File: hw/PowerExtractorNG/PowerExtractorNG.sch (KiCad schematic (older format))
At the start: 11 parts, among them J1 INPUT RECTIFIED, J2 OUTPUT, Q1 IRFB4110

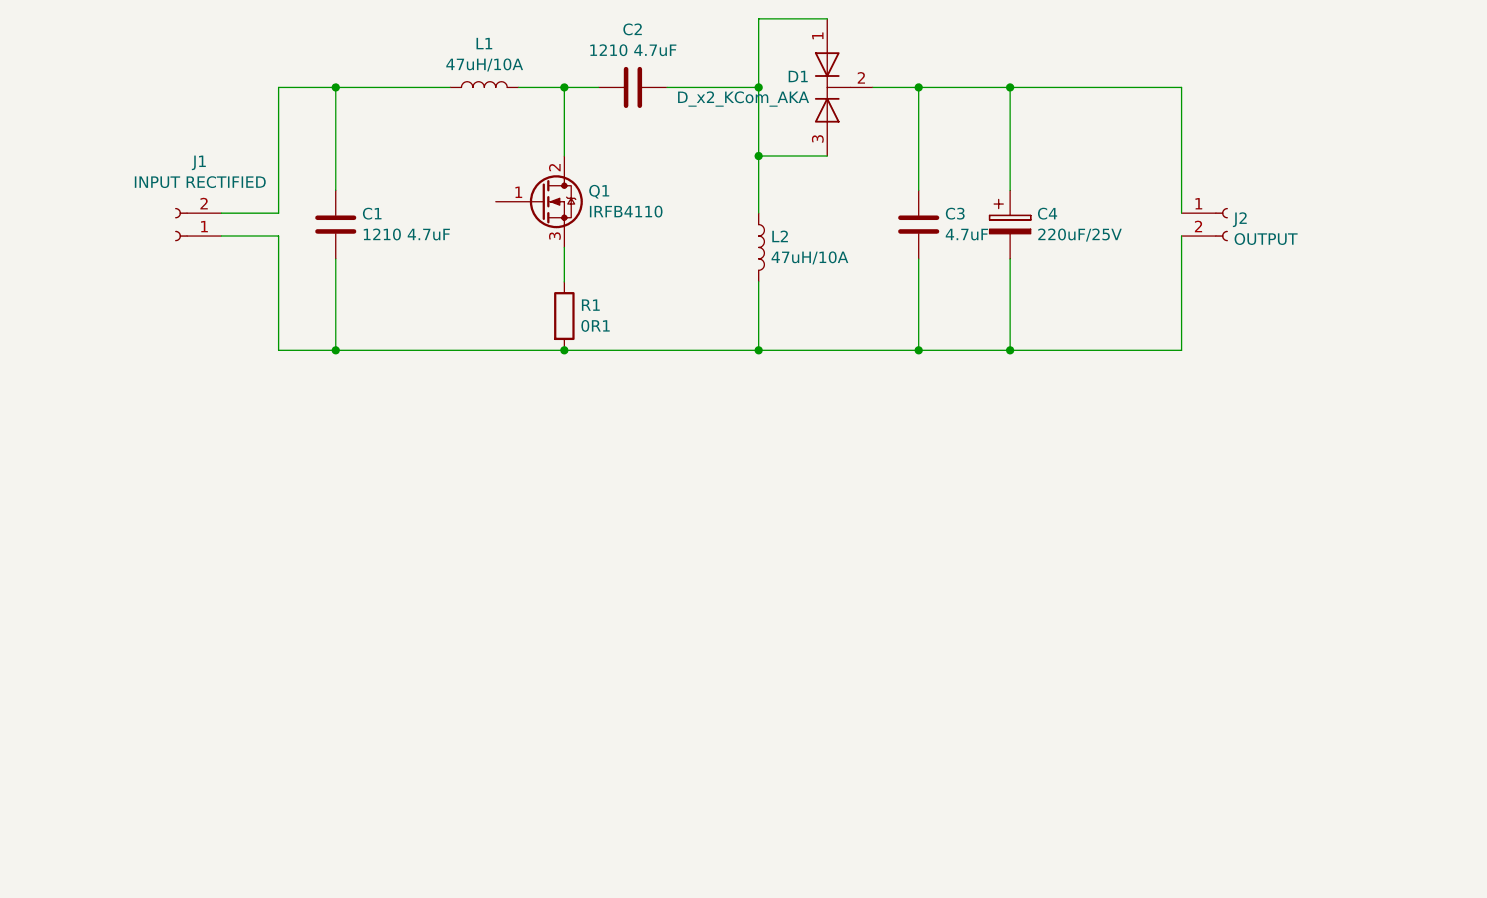
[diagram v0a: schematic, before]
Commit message: Done
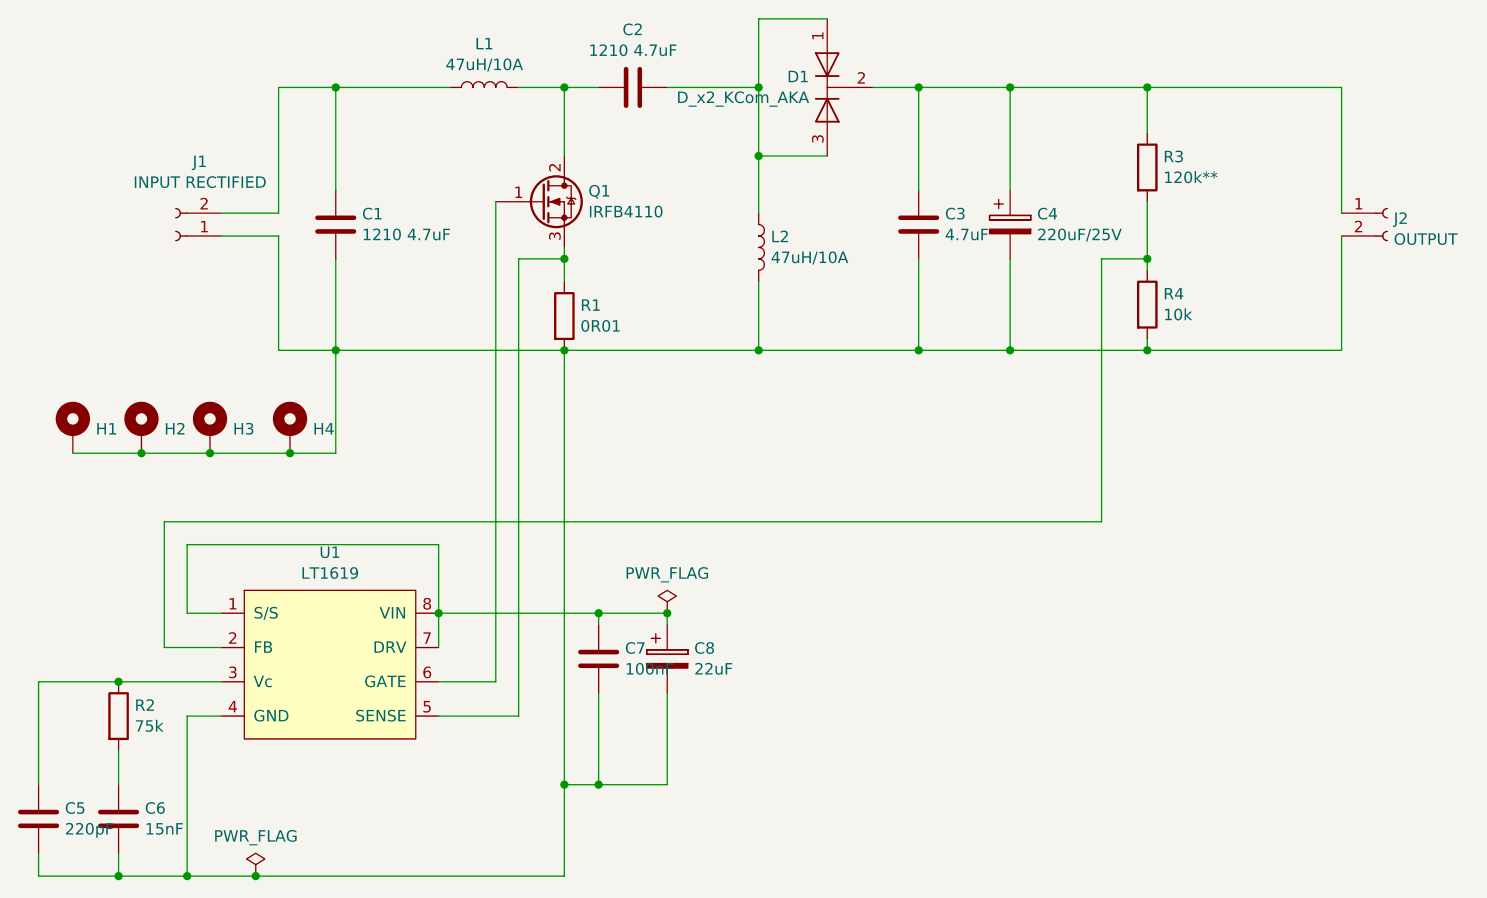
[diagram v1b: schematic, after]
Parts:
- added C5: 220pF, Capacitor_SMD:C_1206_3216Metric_Pad1.42x1.75mm_HandSolder, symbol Device:C
- added C6: 15nF, Capacitor_SMD:C_1206_3216Metric_Pad1.42x1.75mm_HandSolder, symbol Device:C
- added C7: 100nF, Capacitor_SMD:C_1206_3216Metric_Pad1.42x1.75mm_HandSolder, symbol Device:C
- added C8: 22uF, Capacitor_THT:CP_Radial_D7.5mm_P2.50mm, symbol Device:CP
- added H1, H2, H3, H4: MountingHole_Pad, MountingHole:MountingHole_3.2mm_M3_Pad, symbol Mechanical:MountingHole_Pad
- added R2: 75k, Resistor_SMD:R_1206_3216Metric_Pad1.42x1.75mm_HandSolder, symbol Device:R
- added R3: 120k**, Resistor_SMD:R_1206_3216Metric_Pad1.42x1.75mm_HandSolder, symbol Device:R
- added R4: 10k, Resistor_SMD:R_1206_3216Metric_Pad1.42x1.75mm_HandSolder, symbol Device:R
- added U1: LT1619, Package_SO:SO-8_5.3x6.2mm_P1.27mm, symbol triakcz_kicad:LT1619
- C4: footprint Capacitor_THT:C_Rect_L7.2mm_W5.5mm_P5.00mm_FKS2_FKP2_MKS2_MKP2 -> Capacitor_THT:CP_Radial_D10.0mm_P5.00mm
- R1: value 0R1 -> 0R01; footprint Resistor_SMD:R_1206_3216Metric_Pad1.42x1.75mm_HandSolder -> Resistor_SMD:R_2512_6332Metric_Pad1.52x3.35mm_HandSolder
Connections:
- net at C1.2, C3.2, C4.2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: now also C5.2, C6.2, C7.2, C8.2, H1.1, H2.1, H3.1, H4.1, R4.2, U1.4 (GND)
- net at C3.1, C4.1, D1.2 (K)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: now also R3.1
- net at Q1.1 (G): now also U1.6 (GATE)
- net at Q1.3 (S), R1.1: now also U1.5 (SENSE)
- new net: C7.1, C8.1, U1.1 (S/S), U1.7 (DRV), U1.8 (VIN)
- new net: R3.2, R4.1, U1.2 (FB)
- new net: C5.1, R2.1, U1.3 (Vc)
- new net: C6.1, R2.2
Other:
- moved on the sheet: J2

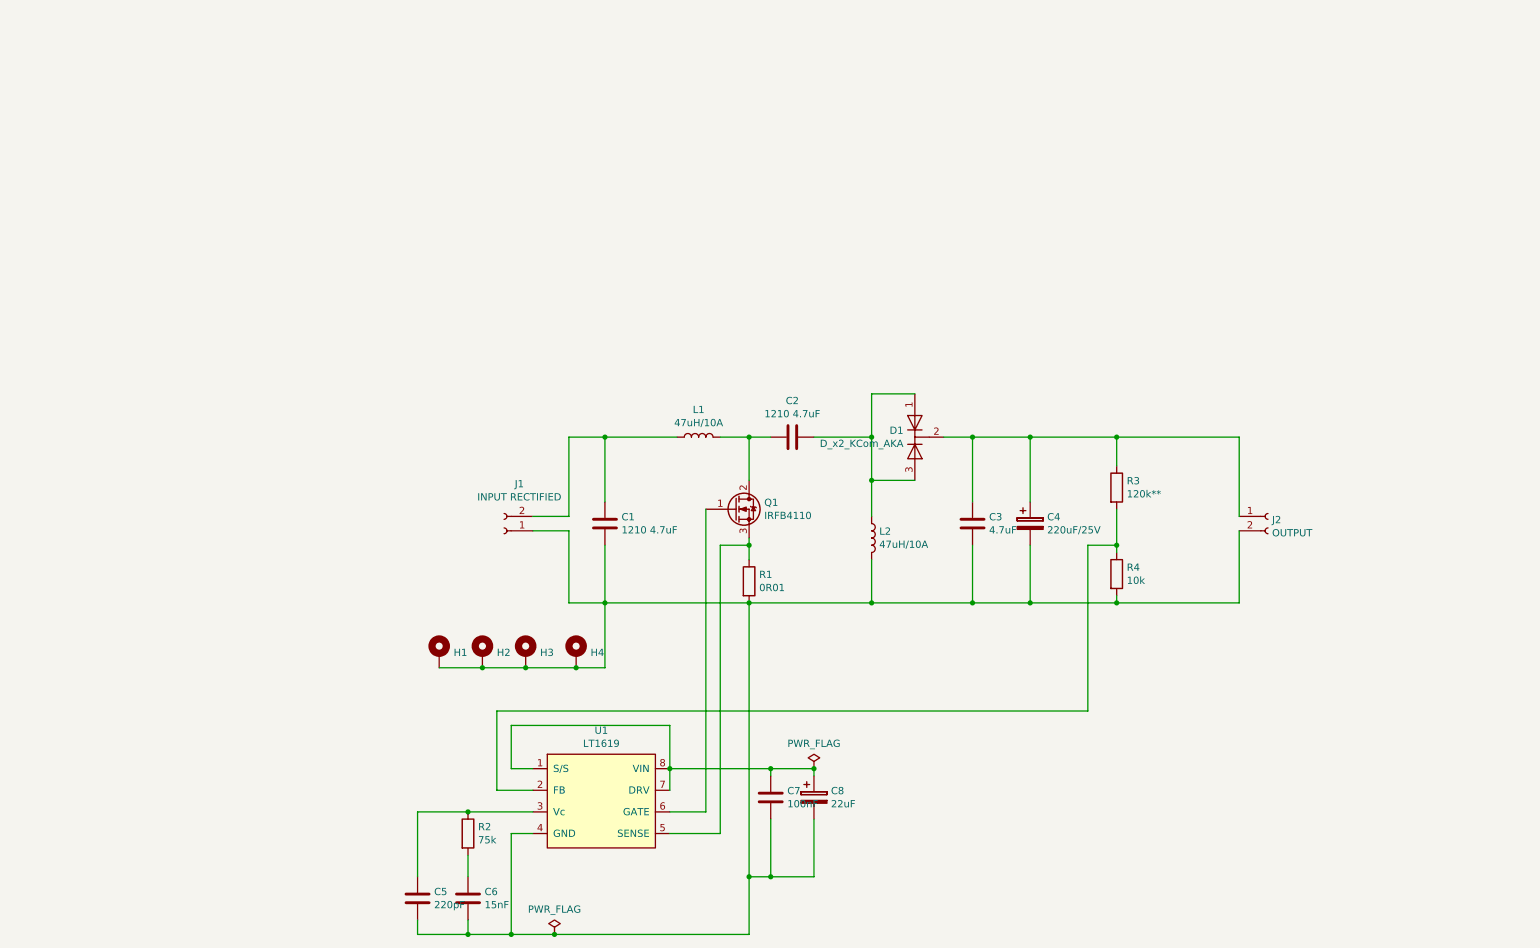
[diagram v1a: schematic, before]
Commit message: PE2020
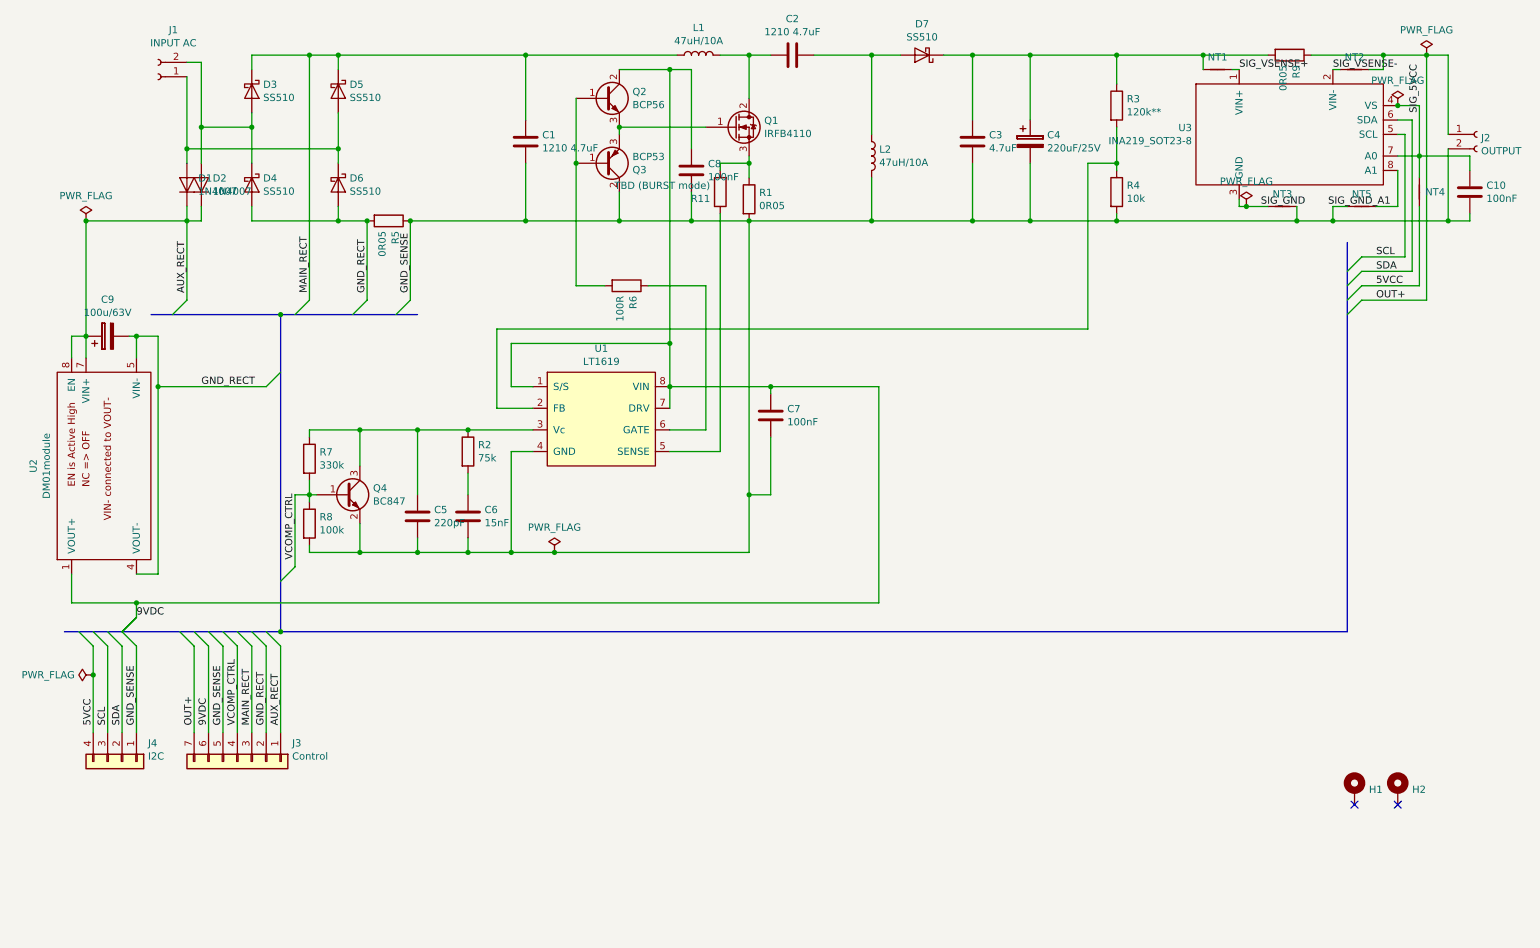
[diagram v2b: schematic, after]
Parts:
- removed C8: 22uF, Capacitor_THT:CP_Radial_D7.5mm_P2.50mm, symbol Device:CP
- removed D1: D_x2_KCom_AKA, Package_TO_SOT_THT:TO-220-3_Vertical, symbol Device:D_x2_KCom_AKA
- removed H3, H4: MountingHole_Pad, MountingHole:MountingHole_3.2mm_M3_Pad, symbol Mechanical:MountingHole_Pad
- added C10, C8: 100nF, Capacitor_SMD:C_1206_3216Metric_Pad1.42x1.75mm_HandSolder, symbol Device:C
- added C9: 100u/63V, Capacitor_THT:CP_Radial_D10.0mm_P5.00mm, symbol Device:CP
- added D1, D2: 1N4007, Diode_SMD:D_SMA, symbol Device:D
- added D3, D4, D5, D6, D7: SS510, Diode_SMD:D_SMC_Handsoldering, symbol Device:D_Schottky
- added J3: Control, Connector_PinHeader_2.54mm:PinHeader_1x07_P2.54mm_Vertical, symbol Connector_Generic:Conn_01x07
- added J4: I2C, Connector_PinHeader_2.54mm:PinHeader_1x04_P2.54mm_Vertical, symbol Connector_Generic:Conn_01x04
- added NT1, NT2, NT3, NT4, NT5: Net-Tie_2, NetTie:NetTie-2_SMD_Pad0.5mm, symbol Device:Net-Tie_2
- added Q2: BCP56, Package_TO_SOT_SMD:SOT-223-3_TabPin2, symbol Device:Q_NPN_BCE
- added Q3: BCP53, Package_TO_SOT_SMD:SOT-223-3_TabPin2, symbol Device:Q_PNP_BCE
- added Q4: BC847, Package_TO_SOT_SMD:SOT-23, symbol Device:Q_NPN_BEC
- added R11: TBD (BURST mode), Resistor_SMD:R_1206_3216Metric_Pad1.42x1.75mm_HandSolder, symbol Device:R
- added R5, R9: 0R05, Resistor_SMD:R_2512_6332Metric_Pad1.52x3.35mm_HandSolder, symbol Device:R
- added R6: 100R, Resistor_SMD:R_1206_3216Metric_Pad1.42x1.75mm_HandSolder, symbol Device:R
- added R7: 330k, Resistor_SMD:R_1206_3216Metric_Pad1.42x1.75mm_HandSolder, symbol Device:R
- added R8: 100k, Resistor_SMD:R_1206_3216Metric_Pad1.42x1.75mm_HandSolder, symbol Device:R
- added U2: DM01module, triakcz_modules:DM01_mod_THT, symbol triakcz_kicad:DM01module
- added U3: INA219_SOT23-8, Package_TO_SOT_SMD:SOT-23-8_Handsoldering, symbol triakcz_kicad:INA219_SOT23-8
- J1: value INPUT RECTIFIED -> INPUT AC
- R1: value 0R01 -> 0R05
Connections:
- net MAIN_RECT: now reaches C1.1, L1.1
- net MAIN_RECT: now also D3.1 (K), D5.1 (K), J3.3 (Pin_3); no longer J1.2 (Pin_2)
- net at C2.1, L2.1: now also D7.2 (A)
- net GND_SENSE: now reaches C1.2, C3.2, C4.2, C5.2, C6.2, C7.2, J2.2 (Pin_2), L2.2, R1.2, R4.2, U1.4 (GND)
- net GND_SENSE: now also C10.2, C8.2, J3.5 (Pin_5), J4.1 (Pin_1), NT3.2, NT5.1, Q3.2 (C), Q4.2 (E), R5.1, R8.2; no longer H1.1, H2.1, J1.1 (Pin_1)
- net at C3.1, C4.1, R3.1: now also D7.1 (K), NT1.1, R9.2; no longer J2.1 (Pin_1)
- net at Q1.1 (G): now also Q2.3 (E), Q3.3 (E); no longer U1.6 (GATE)
- net at Q1.3 (S), R1.1: now also R11.2; no longer U1.5 (SENSE)
- net 9VDC: now reaches C7.1, U1.1 (S/S), U1.7 (DRV), U1.8 (VIN)
- net 9VDC: now also C8.1, J3.6 (Pin_6), Q2.2 (C), U2.1 (VOUT+)
- net at C5.1, R2.1, U1.3 (Vc): now also Q4.3 (C), R7.1
- new net: D1.2 (A), D5.2 (A), D6.1 (K), J1.1 (Pin_1)
- new net: D2.2 (A), D3.2 (A), D4.1 (K), J1.2 (Pin_2)
- new net: R11.1, U1.5 (SENSE)
- new net: R6.1, U1.6 (GATE)
- new net: Q2.1 (B), Q3.1 (B), R6.2
- new net 5VCC: J4.4 (Pin_4), NT4.2
- new net AUX_RECT: C9.1, D1.1 (K), D2.1 (K), J3.1 (Pin_1), U2.7 (VIN+), U2.8 (EN)
- new net GND_RECT: C9.2, D4.2 (A), D6.2 (A), J3.2 (Pin_2), R5.2, U2.4 (VOUT-), U2.5 (VIN-)
- new net OUT+: J2.1 (Pin_1), J3.7 (Pin_7), NT2.2, R9.1
- new net SCL: J4.3 (Pin_3), U3.5 (SCL)
- new net SDA: J4.2 (Pin_2), U3.6 (SDA)
- new net SIG_5VCC: C10.1, NT4.1, U3.4 (VS), U3.7 (A0)
- new net SIG_GND: NT3.1, U3.3 (GND)
- new net SIG_GND_A1: NT5.2, U3.8 (A1)
- new net SIG_VSENSE+: NT1.2, U3.1 (VIN+)
- new net SIG_VSENSE-: NT2.1, U3.2 (VIN-)
- new net VCOMP_CTRL: J3.4 (Pin_4), Q4.1 (B), R7.2, R8.1
- no-connect marks 0 -> 2
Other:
- moved on the sheet: C1, C2, C3, C4, C5, C6, C7, H1, H2, J1, J2, L1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
